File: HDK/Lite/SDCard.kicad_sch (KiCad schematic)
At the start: 1 part, among them J301 GT-TF003-H0185-02

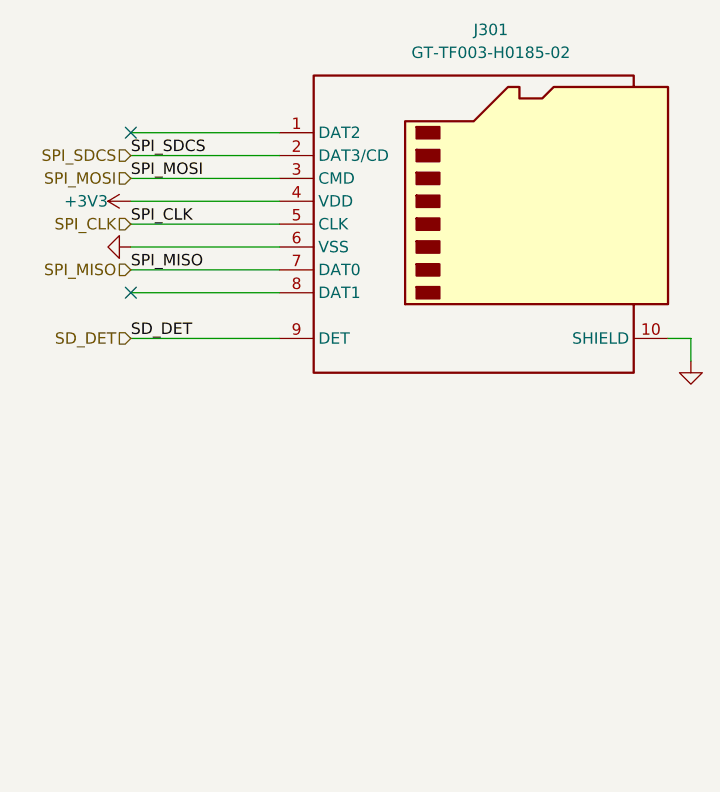
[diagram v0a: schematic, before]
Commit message: updated 1-Job, v1rA
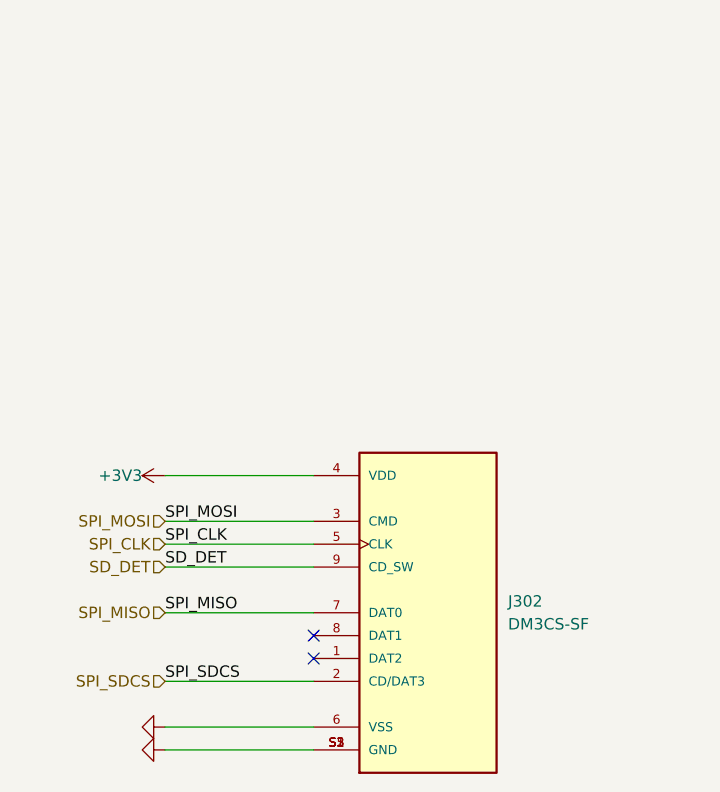
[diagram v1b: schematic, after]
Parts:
- removed J301: GT-TF003-H0185-02, Connector_Card:microSD_HC_Molex_104031-0811, symbol Connector:Micro_SD_Card_Det1
- added J302: DM3CS-SF, footprints:HRS_DM3CS-SF, symbol DM3CS-SF:DM3CS-SF
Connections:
- net +3V3: now also J302.4 (VDD)
- net GND: now also J302.6 (VSS), J302.S1 (GND), J302.S2 (GND), J302.S3 (GND), J302.S5 (GND)
- net SD_DET: now also J302.9 (CD_SW)
- net SPI_CLK: now also J302.5 (CLK)
- net SPI_MISO: now also J302.7 (DAT0)
- net SPI_MOSI: now also J302.3 (CMD)
- net SPI_SDCS: now also J302.2 (CD/DAT3)
